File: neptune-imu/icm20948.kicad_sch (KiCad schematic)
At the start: 3 parts, among them U2 ICM-20948

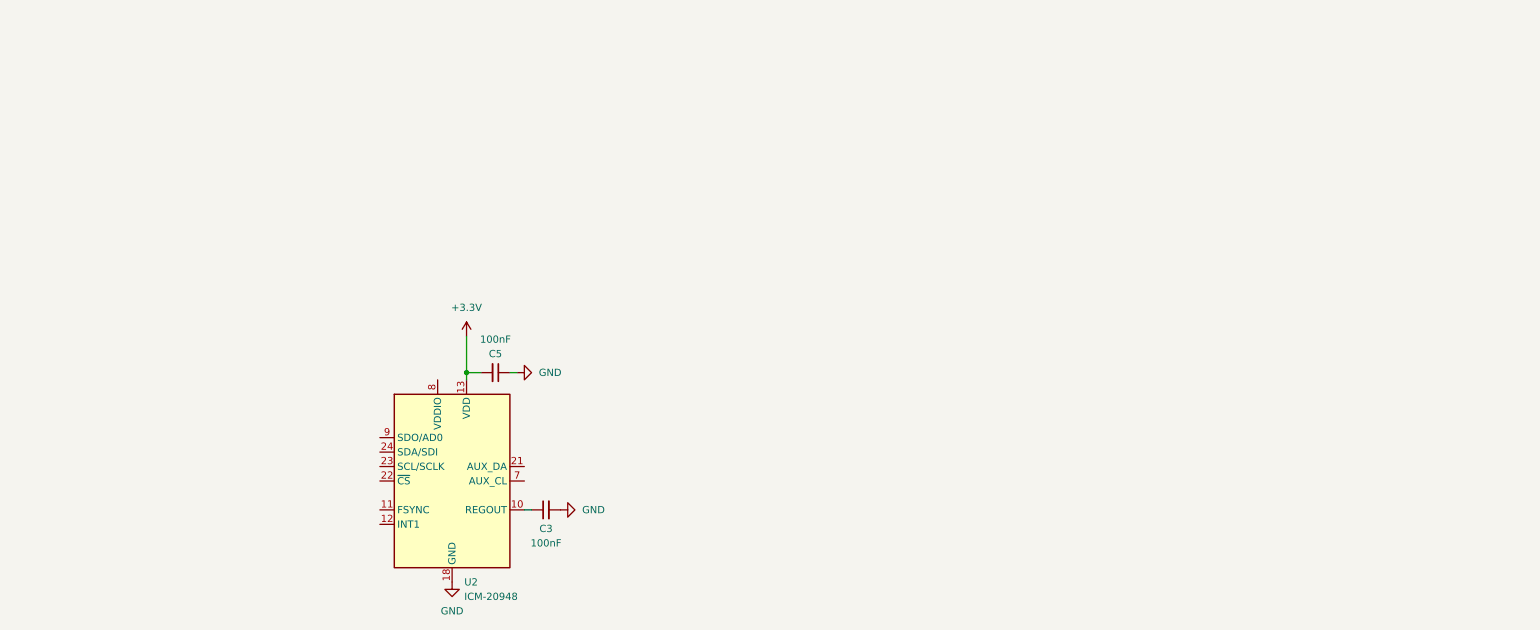
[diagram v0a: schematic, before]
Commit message: session finished
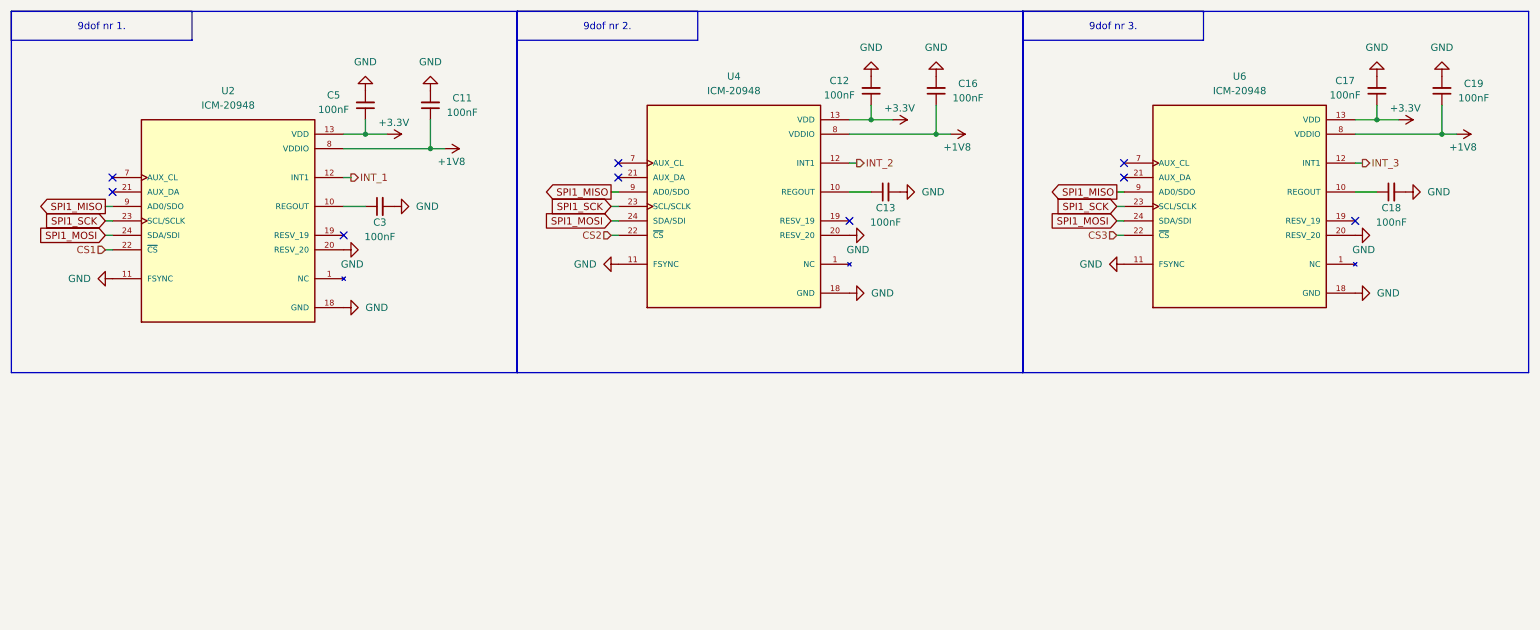
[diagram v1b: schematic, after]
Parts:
- removed U2: ICM-20948, Sensor_Motion:InvenSense_QFN-24_3x3mm_P0.4mm, symbol Sensor_Motion:ICM-20948
- added C11, C12, C13, C16, C17, C18, C19: 100nF, symbol Device:C_Small
- added U2, U4, U6: ICM-20948, ICM-20948:QFN40P300X300X105-24N, symbol neptune-imu-symbols:ICM-20948
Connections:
- net +3.3V: now also C5.1, C12.1, C17.1, U2.13 (VDD), U4.13 (VDD), U6.13 (VDD); no longer C5.2
- net GND: now also C5.2, C11.2, C12.2, C13.2, C16.2, C17.2, C18.2, C19.2, U2.11 (FSYNC), U2.18 (GND), U2.20 (RESV_20), U4.11 (FSYNC), U4.18 (GND), U4.20 (RESV_20), U6.11 (FSYNC), U6.18 (GND), U6.20 (RESV_20); no longer C5.1
- net at C3.1: now also U2.10 (REGOUT)
- new net: C18.1, U6.10 (REGOUT)
- new net: C13.1, U4.10 (REGOUT)
- new net: U2.1 (NC), U2.14 (NC), U2.15 (NC), U2.16 (NC), U2.17 (NC), U2.2 (NC), U2.3 (NC), U2.4 (NC), U2.5 (NC), U2.6 (NC)
- new net: U4.1 (NC), U4.14 (NC), U4.15 (NC), U4.16 (NC), U4.17 (NC), U4.2 (NC), U4.3 (NC), U4.4 (NC), U4.5 (NC), U4.6 (NC)
- new net: U6.1 (NC), U6.14 (NC), U6.15 (NC), U6.16 (NC), U6.17 (NC), U6.2 (NC), U6.3 (NC), U6.4 (NC), U6.5 (NC), U6.6 (NC)
- new net +1V8: C11.1, C16.1, C19.1, U2.8 (VDDIO), U4.8 (VDDIO), U6.8 (VDDIO)
- new net CS1: U2.22 (~{CS})
- new net CS2: U4.22 (~{CS})
- new net CS3: U6.22 (~{CS})
- new net INT_1: U2.12 (INT1)
- new net INT_2: U4.12 (INT1)
- new net INT_3: U6.12 (INT1)
- new net SPI1_MISO: U2.9 (AD0/SDO), U4.9 (AD0/SDO), U6.9 (AD0/SDO)
- new net SPI1_MOSI: U2.24 (SDA/SDI), U4.24 (SDA/SDI), U6.24 (SDA/SDI)
- new net SPI1_SCK: U2.23 (SCL/SCLK), U4.23 (SCL/SCLK), U6.23 (SCL/SCLK)
- no-connect marks 0 -> 9
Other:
- company: (none) -> OnionSAT
- title: (none) -> 9DOF

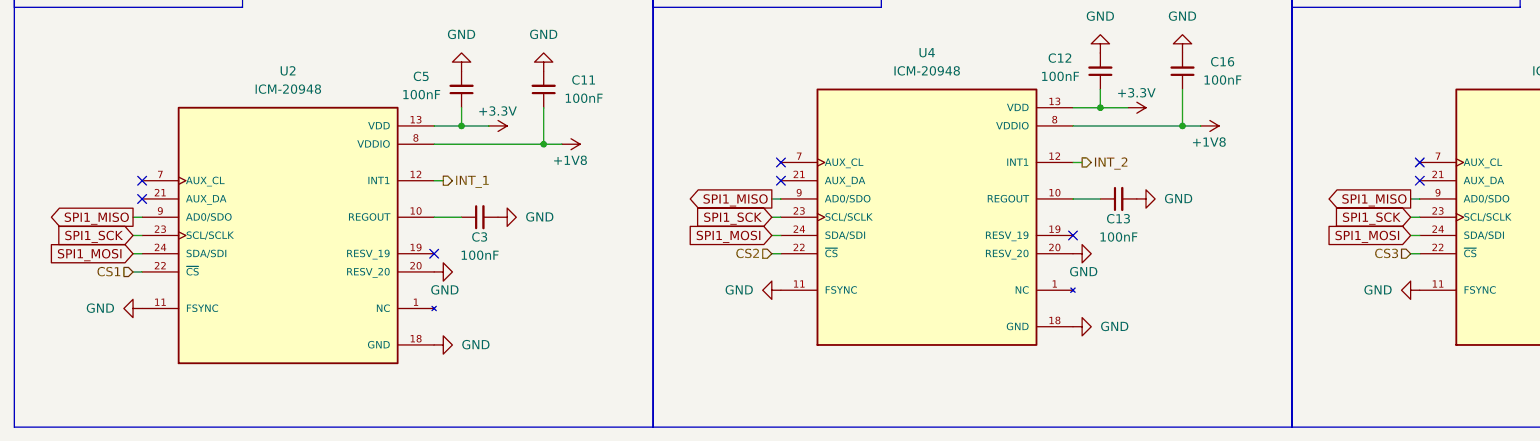
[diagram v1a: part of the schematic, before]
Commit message: Pécsi folytatja a cuccost
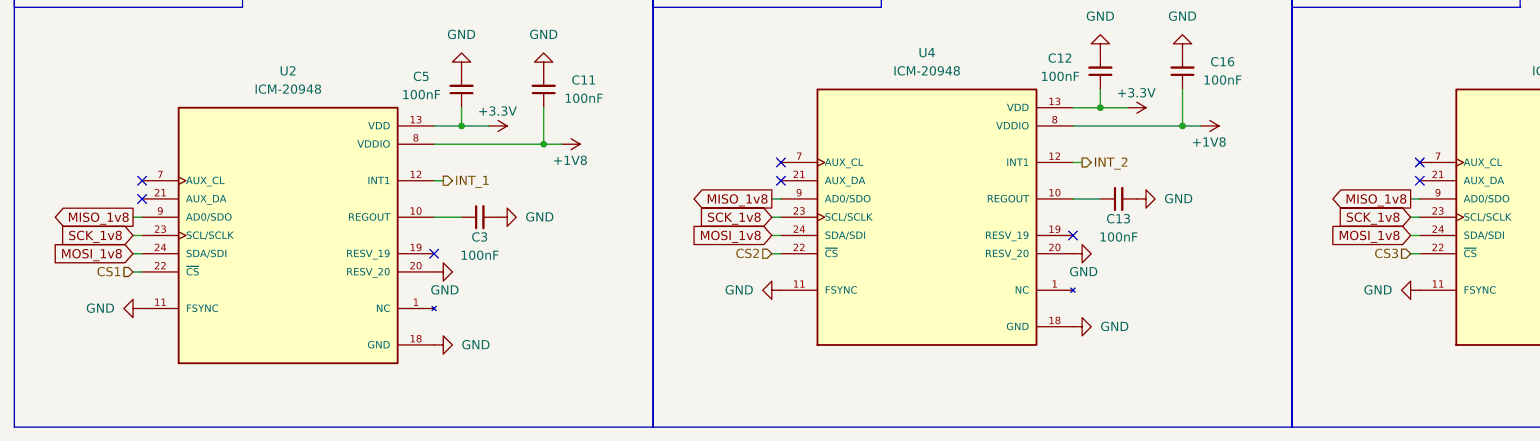
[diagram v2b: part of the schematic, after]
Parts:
- U2, U4, U6: footprint ICM-20948:QFN40P300X300X105-24N -> (none)
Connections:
- net SPI1_MISO renamed MISO_1v8
- net SPI1_MOSI renamed MOSI_1v8
- net SPI1_SCK renamed SCK_1v8
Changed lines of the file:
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@@
 		)
 	)
-	(global_label "SPI1_MOSI"
+	(global_label "MOSI_1v8"
 		(shape input)
 		(at 31.75 55.88 180)
@@
 		)
 		(property "Intersheetrefs" "${INTERSHEET_REFS}"
-			(at 18.9072 55.88 0)
+			(at 19.8144 55.88 0)
 			(effects
 				(font
@@
 		)
 	)
-	(global_label "SPI1_SCK"
+	(global_label "SCK_1v8"
 		(shape input)
 		(at 120.65 50.8 180)
@@
 		)
 		(property "Intersheetrefs" "${INTERSHEET_REFS}"
-			(at 108.6539 50.8 0)
+			(at 109.5611 50.8 0)
 			(effects
 				(font
@@
 		)
 	)
-	(global_label "SPI1_SCK"
+	(global_label "SCK_1v8"
 		(shape input)
 		(at 209.55 50.8 180)
@@
 		)
 		(property "Intersheetrefs" "${INTERSHEET_REFS}"
-			(at 197.5539 50.8 0)
+			(at 198.4611 50.8 0)
 			(effects
 				(font
@@
 		)
 	)
-	(global_label "SPI1_MISO"
+	(global_label "MISO_1v8"
 		(shape output)
 		(at 209.55 48.26 180)
@@
 		)
 		(property "Intersheetrefs" "${INTERSHEET_REFS}"
-			(at 196.7072 48.26 0)
+			(at 197.6144 48.26 0)
 			(effects
 				(font
@@
 		)
 	)
-	(global_label "SPI1_MISO"
+	(global_label "MISO_1v8"
 		(shape output)
 		(at 120.65 48.26 180)
@@
 		)
 		(property "Intersheetrefs" "${INTERSHEET_REFS}"
-			(at 107.8072 48.26 0)
+			(at 108.7144 48.26 0)
 			(effects
 				(font
@@
 		)
 	)
-	(global_label "SPI1_MISO"
+	(global_label "MISO_1v8"
 		(shape output)
 		(at 31.75 50.8 180)
@@
 		)
 		(property "Intersheetrefs" "${INTERSHEET_REFS}"
-			(at 18.9072 50.8 0)
+			(at 19.8144 50.8 0)
 			(effects
 				(font
@@
 		)
 	)
-	(global_label "SPI1_MOSI"
+	(global_label "MOSI_1v8"
 		(shape input)
 		(at 209.55 53.34 180)
@@
 		)
 		(property "Intersheetrefs" "${INTERSHEET_REFS}"
-			(at 196.7072 53.34 0)
+			(at 197.6144 53.34 0)
 			(effects
 				(font
@@
 		)
 	)
-	(global_label "SPI1_SCK"
+	(global_label "SCK_1v8"
 		(shape input)
 		(at 31.75 53.34 180)
@@
 		)
 		(property "Intersheetrefs" "${INTERSHEET_REFS}"
-			(at 19.7539 53.34 0)
+			(at 20.6611 53.34 0)
 			(effects
 				(font
@@
 		)
 	)
-	(global_label "SPI1_MOSI"
+	(global_label "MOSI_1v8"
 		(shape input)
 		(at 120.65 53.34 180)
@@
 		)
 		(property "Intersheetrefs" "${INTERSHEET_REFS}"
-			(at 107.8072 53.34 0)
+			(at 108.7144 53.34 0)
 			(effects
 				(font
@@
 			)
 		)
-		(property "Footprint" "ICM-20948:QFN40P300X300X105-24N"
+		(property "Footprint" ""
 			(at 53.34 53.34 0)
 			(effects
@@
 			)
 		)
-		(property "Footprint" "ICM-20948:QFN40P300X300X105-24N"
+		(property "Footprint" ""
 			(at 142.24 50.8 0)
 			(effects
@@
 			)
 		)
-		(property "Footprint" "ICM-20948:QFN40P300X300X105-24N"
+		(property "Footprint" ""
 			(at 231.14 50.8 0)
 			(effects
